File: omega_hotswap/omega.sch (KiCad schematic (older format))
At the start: 61 parts, among them SW1 SW_Push, U1 ProMicro

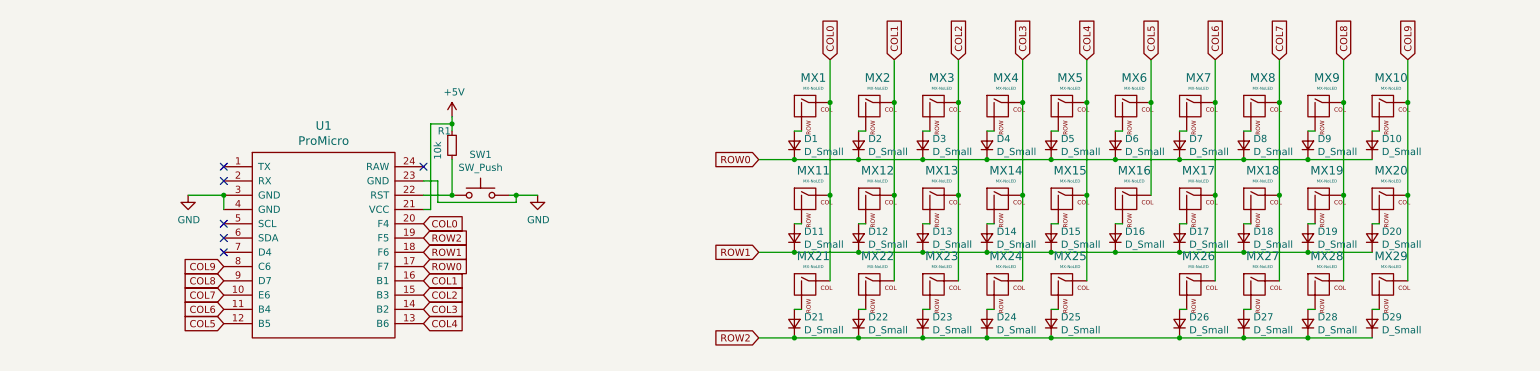
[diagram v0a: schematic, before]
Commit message: work
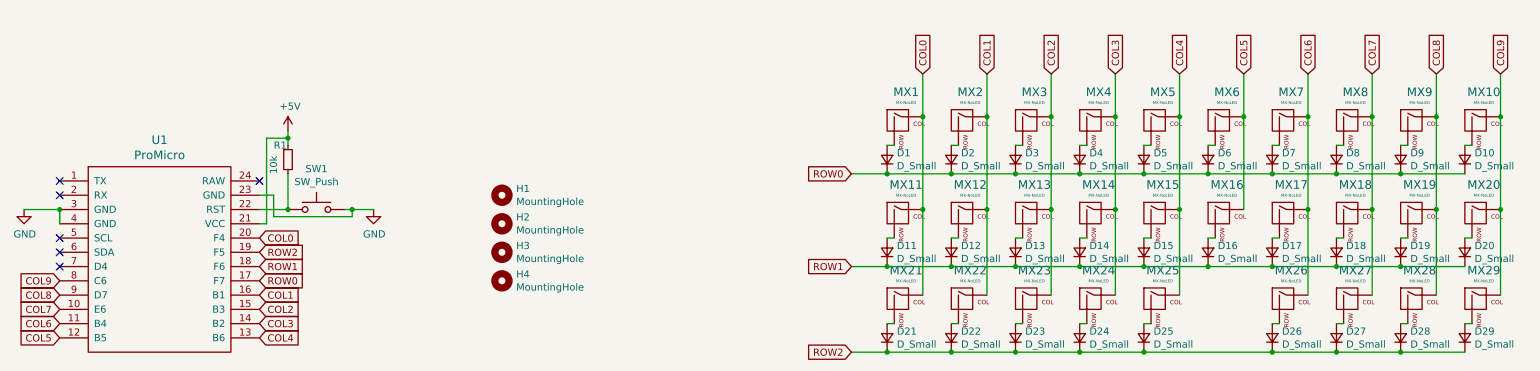
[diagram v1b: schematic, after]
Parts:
- added H1, H2, H3, H4: MountingHole, MountingHole:MountingHole_2.2mm_M2_Pad, symbol Mechanical:MountingHole
- D1, D10, D11, D12, D13, D14, D15, D16, D17, D18, D19, D2, D20, D21, D22, D23, D24, D25, D26, D27, D28, D29, D3, D4, D5, D6, D7, D8, D9: footprint Diode_THT:D_DO-35_SOD27_P3.81mm_Vertical_AnodeUp -> Keebio-Parts:Diode-Hybrid-Back
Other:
- moved on the sheet: D1, D10, D11, D12, D13, D14, D15, D16, D17, D18, D19, D2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
